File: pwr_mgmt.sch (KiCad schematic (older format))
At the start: 26 parts

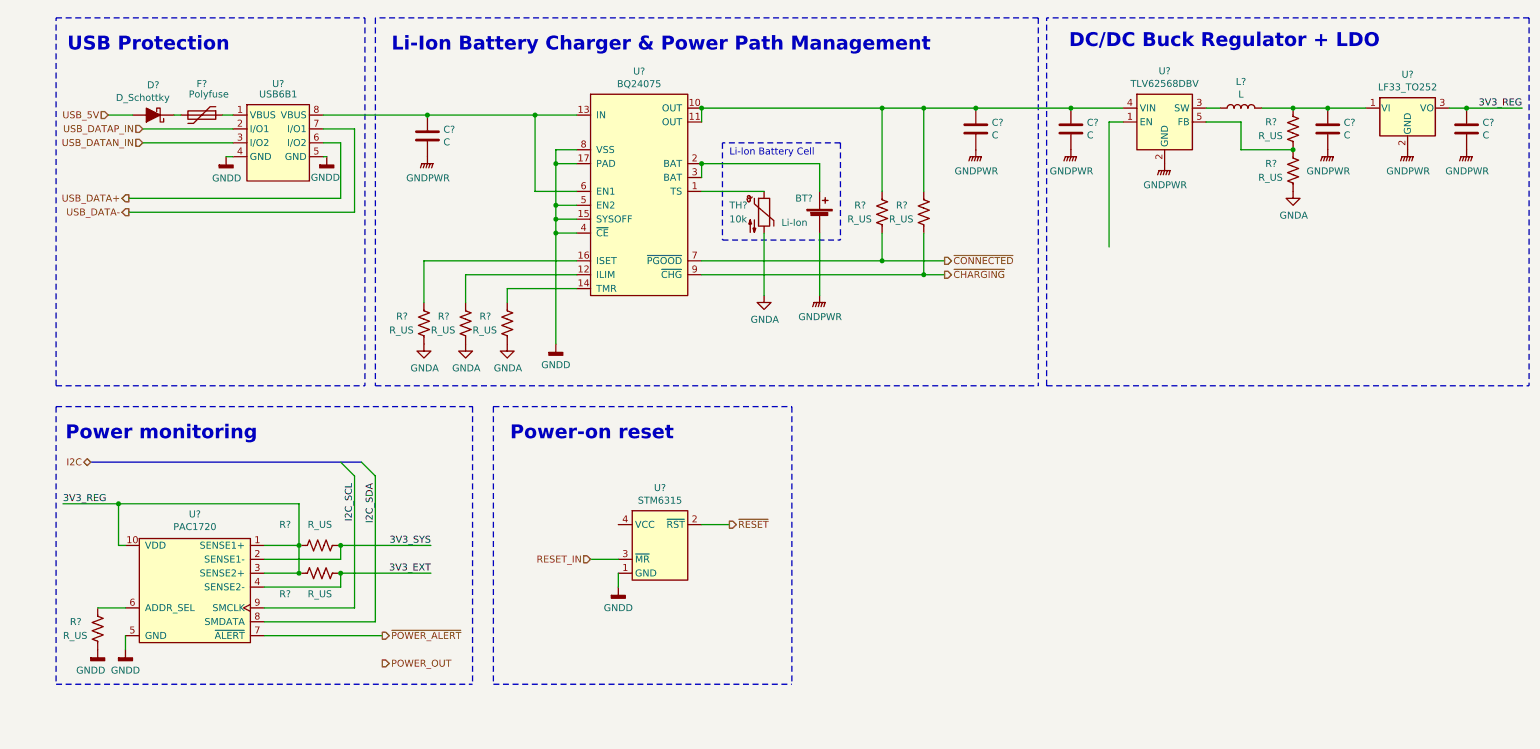
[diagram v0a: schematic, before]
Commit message: Power management & Documentation updates, source includes
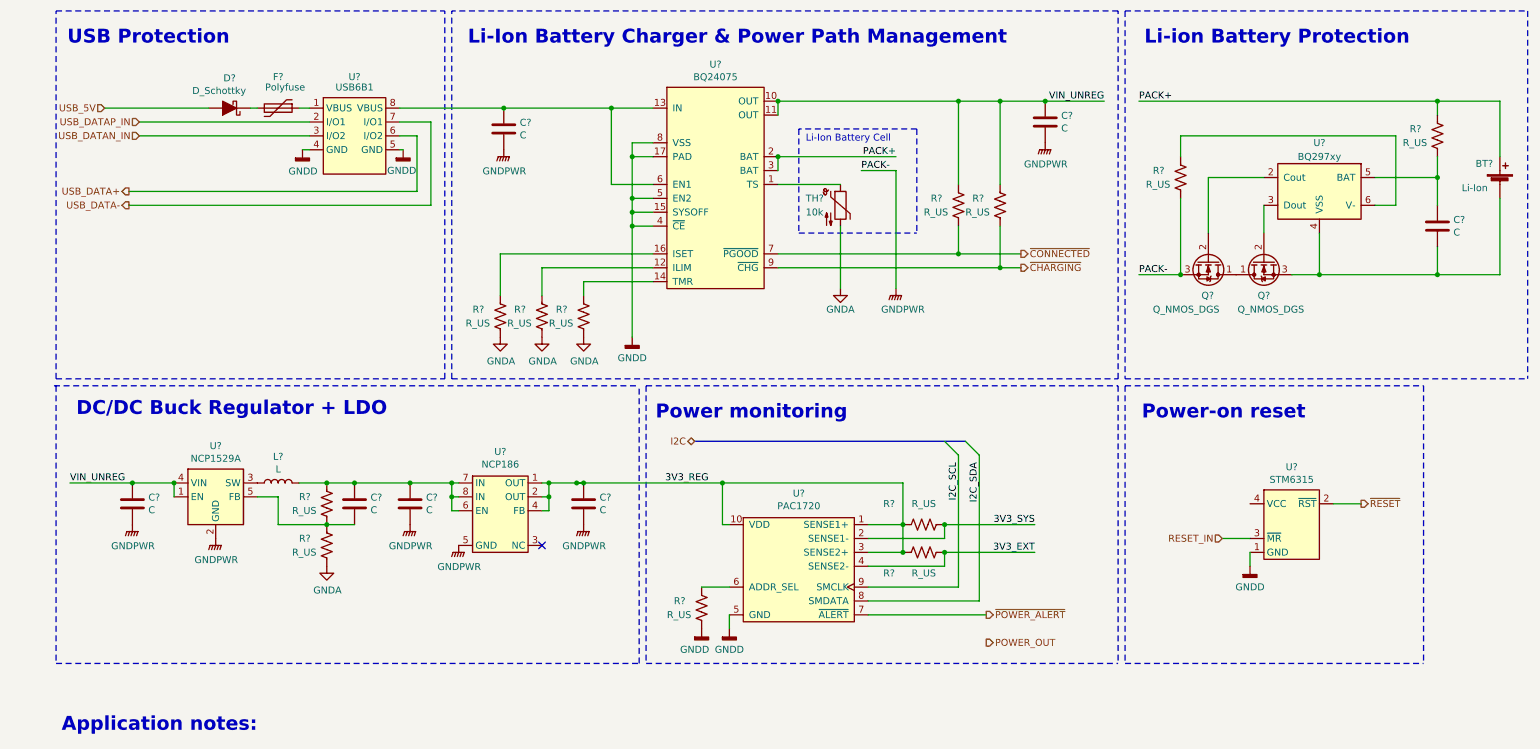
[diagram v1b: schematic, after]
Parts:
- removed BT?: Li-Ion, symbol Device:Battery_Cell
- removed C? (x2): C, symbol Device:C
- removed D?: D_Schottky, symbol Device:D_Schottky_ALT
- removed L?: L, symbol Device:L
- removed R? (x2): R_US, symbol Device:R_US
- removed U?: TLV62568DBV, Package_TO_SOT_SMD:SOT-23-5, symbol Regulator_Switching:TLV62568DBV
- removed U?: LF33_TO252, Package_TO_SOT_SMD:TO-252-2, symbol Regulator_Linear:LF33_TO252
- added BT?: Li-Ion, symbol Device:Battery_Cell
- added C? (x4): C, symbol Device:C
- added D?: D_Schottky, symbol Device:D_Schottky_ALT
- added L?: L, symbol Device:L
- added Q? (x2): Q_NMOS_DGS, symbol Device:Q_NMOS_DGS
- added R? (x4): R_US, symbol Device:R_US
- added U?: BQ297xy, Package_SON:WSON-6_1.5x1.5mm_P0.5mm, symbol Battery_Management:BQ297xy
- added U?: NCP186, symbol Regulator_Linear:NCP186
- added U?: NCP1529A, Package_TO_SOT_SMD:SOT-23-5, symbol Regulator_Switching:NCP1529A
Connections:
- net 3V3_REG: now also U?.1 (OUT), U?.2 (OUT), U?.4 (FB)
- net GNDA: now also R?.2
- net GNDPWR: now also C?.2, C?.2, Q?.3 (S), R?.2, U?.2 (GND), U?.5 (GND)
- net USB_5V: now also D?.2 (A)
- net at F?.2: now also D?.1 (K)
- net VIN_UNREG: now reaches C?.1, R?.1, R?.1, U?.10 (OUT), U?.11 (OUT)
- net VIN_UNREG: now also C?.1, U?.1 (EN), U?.4 (VIN)
- net PACK+: now reaches U?.2 (BAT), U?.3 (BAT)
- net PACK+: now also BT?.1 (+), R?.1
- new net: Q?.2 (G), U?.2 (Cout)
- new net: Q?.2 (G), U?.3 (Dout)
- new net: BT?.2 (-), C?.2, Q?.3 (S), U?.4 (VSS)
- new net: C?.1, R?.2, U?.5 (BAT)
- new net: R?.1, U?.6 (V-)
- new net: Q?.1 (D), Q?.1 (D)
- new net: C?.1, C?.1, L?.2, R?.1, U?.6 (EN), U?.7 (IN), U?.8 (IN)
- new net: L?.1, U?.3 (SW)
- new net: C?.2, R?.1, R?.2, U?.5 (FB)
- no-connect marks 0 -> 1
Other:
- note added: "Application notes:"
- note added: "Li-ion Battery Protection"
- moved on the sheet: C?, F?, R?, TH?, U?
